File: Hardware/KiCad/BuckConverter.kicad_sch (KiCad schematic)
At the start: 12 parts, among them U1 TPS56339DDC

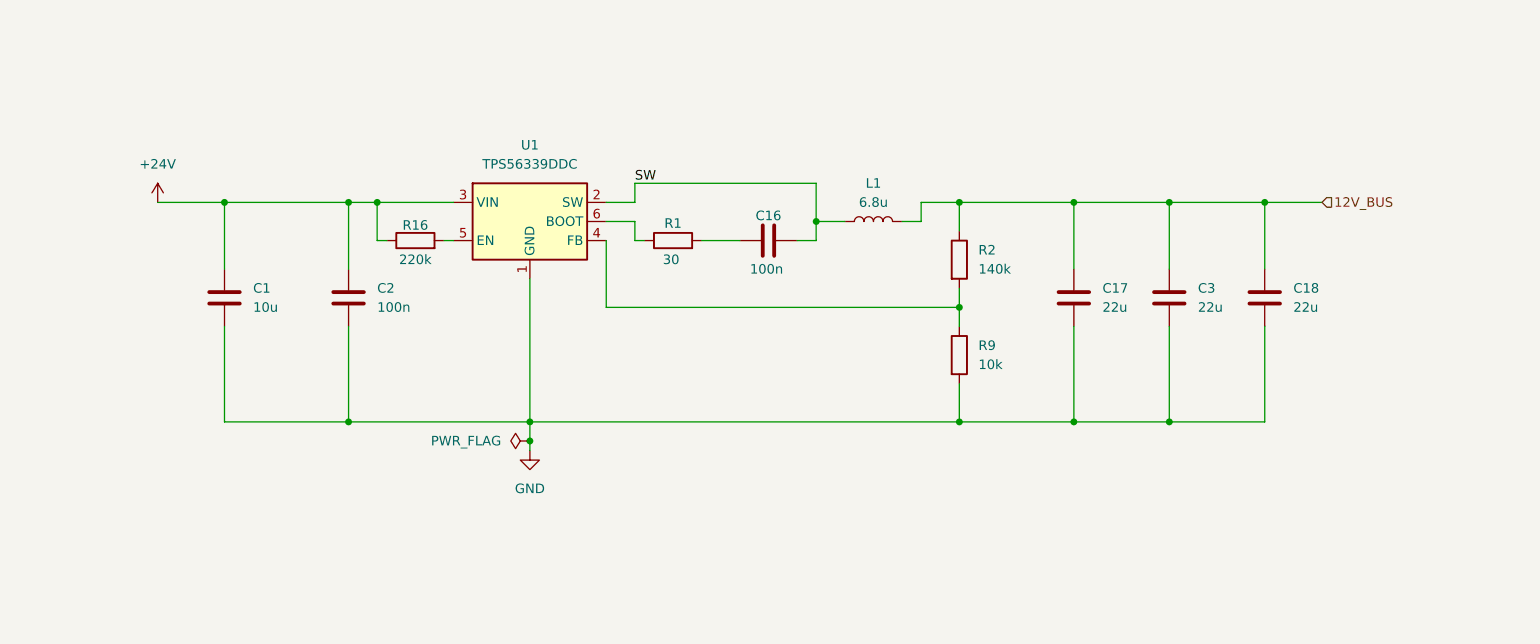
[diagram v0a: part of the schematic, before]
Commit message: revB
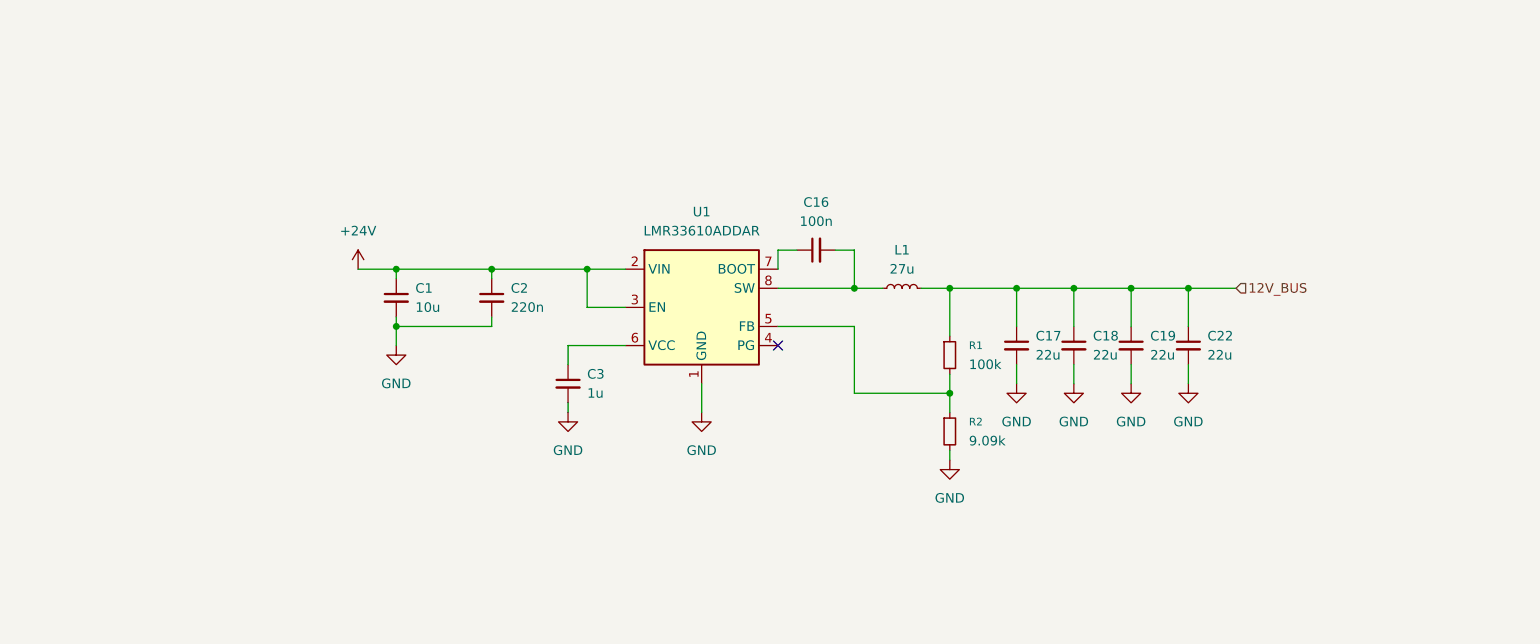
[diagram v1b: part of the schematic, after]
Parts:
- removed C1: 10u, Capacitor_SMD:C_0805_2012Metric_Pad1.18x1.45mm_HandSolder, symbol Device:C
- removed C16, C2: 100n, Capacitor_SMD:C_0603_1608Metric_Pad1.08x0.95mm_HandSolder, symbol Device:C
- removed C17, C18, C3: 22u, Capacitor_SMD:C_0805_2012Metric_Pad1.18x1.45mm_HandSolder, symbol Device:C
- removed L1: 6.8u, Inductor_SMD:L_6.3x6.3_H3, symbol Device:L
- removed R1: 30, Resistor_SMD:R_0603_1608Metric_Pad0.98x0.95mm_HandSolder, symbol Device:R
- removed R16: 220k, Resistor_SMD:R_0603_1608Metric_Pad0.98x0.95mm_HandSolder, symbol Device:R
- removed R2: 140k, Resistor_SMD:R_0603_1608Metric_Pad0.98x0.95mm_HandSolder, symbol Device:R
- removed R9: 10k, Resistor_SMD:R_0603_1608Metric_Pad0.98x0.95mm_HandSolder, symbol Device:R
- removed U1: TPS56339DDC, Package_TO_SOT_SMD:SOT-23-6, symbol Regulator_Switching:TPS56339DDC
- added C1: 10u, Capacitor_SMD:C_0805_2012Metric_Pad1.18x1.45mm_HandSolder, symbol Device:C_Small
- added C16: 100n, Capacitor_SMD:C_0603_1608Metric_Pad1.08x0.95mm_HandSolder, symbol Device:C_Small
- added C17, C18, C19, C22: 22u, Capacitor_SMD:C_0805_2012Metric_Pad1.18x1.45mm_HandSolder, symbol Device:C_Small
- added C2: 220n, Capacitor_SMD:C_0603_1608Metric_Pad1.08x0.95mm_HandSolder, symbol Device:C_Small
- added C3: 1u, Capacitor_SMD:C_0603_1608Metric_Pad1.08x0.95mm_HandSolder, symbol Device:C_Small
- added L1: 27u, symbol Device:L_Small
- added R1: 100k, Resistor_SMD:R_0603_1608Metric_Pad0.98x0.95mm_HandSolder, symbol Device:R_Small
- added R2: 9.09k, Resistor_SMD:R_0603_1608Metric_Pad0.98x0.95mm_HandSolder, symbol Device:R_Small
- added U1: LMR33610ADDAR, Package_SO:Texas_HSOP-8-1EP_3.9x4.9mm_P1.27mm_ThermalVias, symbol Regulator_Switching:LMR33610ADDAR
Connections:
- net +24V: now also C1.1, C2.1, U1.2 (VIN), U1.3 (EN)
- net 12V_BUS: now also C17.1, C18.1, C19.1, C22.1, L1.2, R1.1
- net GND: now also C1.2, C17.2, C18.2, C19.2, C2.2, C22.2, C3.2, R2.2, U1.1 (GND), U1.9 (GND)
- new net: R1.2, R2.1, U1.5 (FB)
- new net: C16.2, L1.1, U1.8 (SW)
- new net: C16.1, U1.7 (BOOT)
- new net: C3.1, U1.6 (VCC)
- no-connect marks 0 -> 1
